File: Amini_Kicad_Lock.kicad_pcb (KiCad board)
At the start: 2 copper layers, 36 parts, among them U1 nRF5340-QKxx, X1 32MHz, X2 32.768kHz

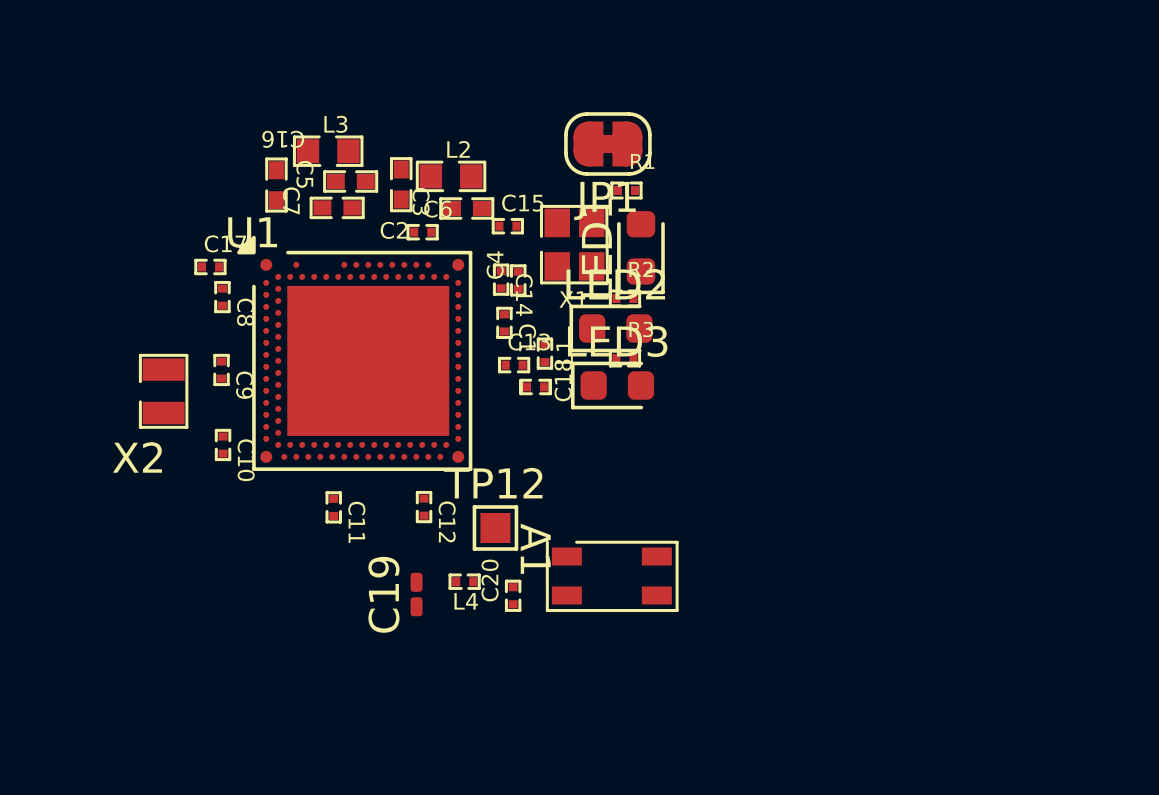
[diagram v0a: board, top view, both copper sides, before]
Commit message: 2. commit
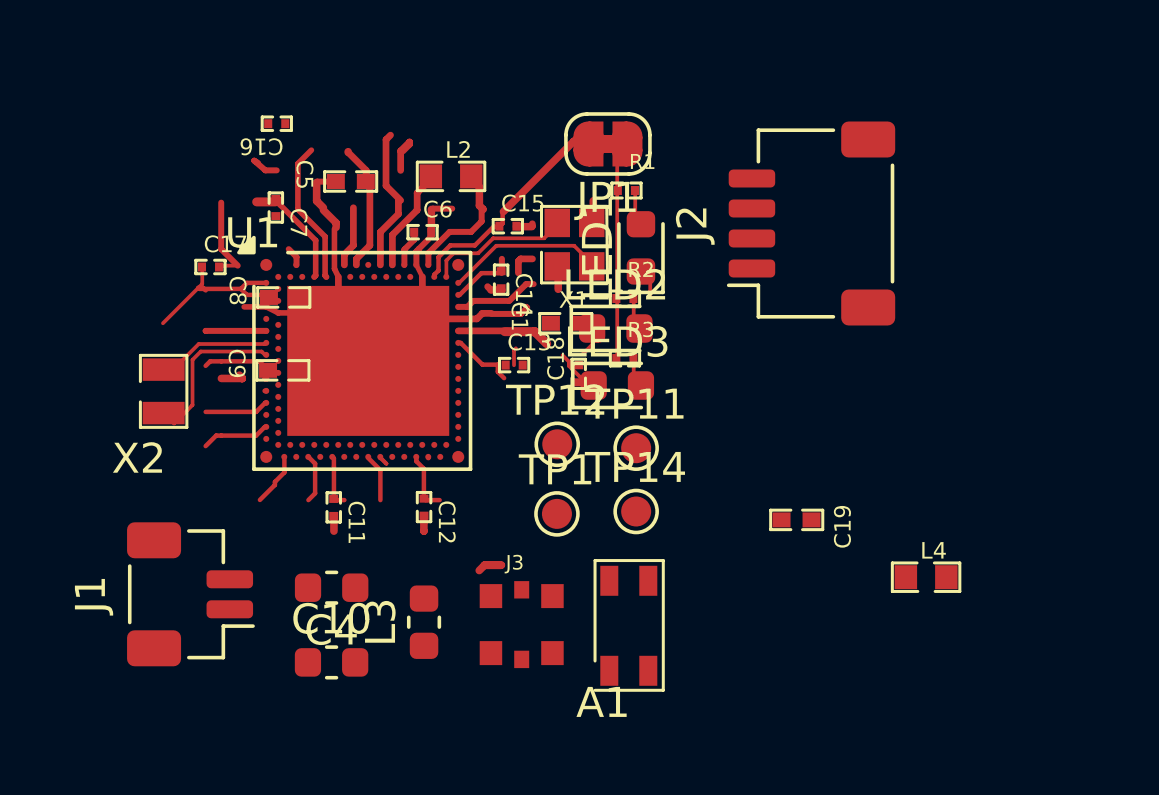
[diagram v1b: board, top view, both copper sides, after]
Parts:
- removed C2, C3: 1.0µF, Nordic_Semiconductor:CAPC1005X04L
- removed C20: 0.5pF, Nordic_Semiconductor:CAPC0603X03L_C
- removed L1: 2.2nH, Nordic_Semiconductor:INDC0603X03L_C
- added J1: Conn_01x02, Connector_JST:JST_SH_BM02B-SRSS-TB_1x02-1MP_P1.00mm_Vertical, F.Cu at (110.8, 74.4)
- added J2: Conn_01x04, Connector_JST:JST_SH_SM04B-SRSS-TB_1x04-1MP_P1.00mm_Horizontal, F.Cu at (131.5, 62.0)
- added J3: MM8130-2600RA2, MM8130-2600RA2 antenna:MURATA_MM8130-2600RA2, F.Cu at (121.9, 75.4)
- added TP1: TestPoint, TestPoint:TestPoint_Pad_D1.0mm, F.Cu at (123.0, 71.7)
- added TP11: TestPoint, TestPoint:TestPoint_Pad_D1.0mm, F.Cu at (125.7, 69.5)
- added TP14: TestPoint, TestPoint:TestPoint_Pad_D1.0mm, F.Cu at (125.7, 71.6)
- C1: value 0.7pF -> 1.0µF; footprint Nordic_Semiconductor:CAPC0603X03L_C -> Nordic_Semiconductor:CAPC1005X04L
- C10: value 100nF -> 0.7pF; footprint Nordic_Semiconductor:CAPC0603X03L_C -> Inductor_SMD:L_0603_1608Metric
- C16: value 1.0µF -> 100nF; footprint Nordic_Semiconductor:CAPC1005X04L -> Nordic_Semiconductor:CAPC0603X03L_C
- C18: value N.C. -> 100nF; footprint Nordic_Semiconductor:CAPC0603X03L_C_NC -> Nordic_Semiconductor:CAPC0603X03L_C
- C19: value N.C. -> 1.0µF; footprint Capacitor_SMD:C_0201_0603Metric_Pad0.64x0.40mm_HandSolder -> Nordic_Semiconductor:CAPC1005X04L
- C4: value 2.2nF -> N.C.; footprint Nordic_Semiconductor:CAPC0603X03L_C -> Inductor_SMD:L_0603_1608Metric
- C7: value 1.0µF -> 2.2nF; footprint Nordic_Semiconductor:CAPC1005X04L -> Nordic_Semiconductor:CAPC0603X03L_C
- C8, C9: value 100nF -> 1.0µF; footprint Nordic_Semiconductor:CAPC0603X03L_C -> Nordic_Semiconductor:CAPC1005X04L
- L3: value 10µH -> 2.2nH; footprint Nordic_Semiconductor:INDC1608X06L -> Inductor_SMD:L_0603_1608Metric
- L4: value 3.3nH -> 10µH; footprint Nordic_Semiconductor:INDC0603X03L_C -> Nordic_Semiconductor:INDC1608X06L
- TP12: footprint TestPoint:TestPoint_Pad_1.0x1.0mm -> TestPoint:TestPoint_Pad_D1.0mm
- moved L4 15.6 mm to (135.6, 74.9)
- moved L3 14.9 mm to (118.6, 75.3), turned to 90 degrees
- moved C19 14.9 mm to (133.1, 72.1)
- moved C4 11.8 mm to (115.5, 74.2), turned to 180 degrees
- moved C10 8.29 mm to (115.5, 76.7), turned to 0 degrees
- moved A1 6.24 mm to (124.6, 78.5), turned to 0 degrees
- moved TP12 3.47 mm to (123.0, 69.4)
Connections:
- C1 pad 1: GND -> VDD_nRF
- C1 pad 2: Net-(U1-ANT) -> GND
- C10 pad 1: VDD_nRF -> GND
- C10 pad 2: GND -> Net-(U1-ANT)
- C16 pad 1: GND -> VDD_nRF
- C16 pad 2: VDD_nRF -> GND
- C18 pad 1: GND -> VDD_nRF
- C18 pad 2: (no net) -> GND
- C19 pad 2: (no net) -> VDD_nRF
- C4 pad 1: Net-(U1-DECR) -> GND
- C4 pad 2: GND -> Net-(C4-Pad2)
- C5 pad 2: Net-(U1-DECD) -> Net-(U1-DECR)
- C7 pad 1: GND -> Net-(U1-DECR)
- C7 pad 2: Net-(U1-DECA) -> GND
- C8 pad 1: VDD_nRF -> GND
- C8 pad 2: GND -> Net-(U1-DECD)
- C9 pad 1: VDD_nRF -> GND
- C9 pad 2: GND -> Net-(U1-DECA)
- L3 pad 1: Net-(U1-DECD) -> Net-(U1-ANT)
- L3 pad 2: Net-(U1-DCCD) -> Net-(C4-Pad2)
- L4 pad 1: Net-(A1-Pad1) -> Net-(U1-DECD)
- L4 pad 2: (no net) -> Net-(U1-DCCD)
- TP12 pad 1: (no net) -> /SWDIO
- U1 pad AK10: (no net) -> unconnected-(U1-IO2/P0.15-PadAK10)
- U1 pad AK12: (no net) -> unconnected-(U1-SCK/P0.17-PadAK12)
- U1 pad AK14: (no net) -> unconnected-(U1-CSN/P0.18-PadAK14)
- U1 pad AK30: (no net) -> unconnected-(U1-AIN6/P0.27-PadAK30)
- U1 pad AK8: (no net) -> unconnected-(U1-IO1/P0.14-PadAK8)
- U1 pad AL27: (no net) -> unconnected-(U1-P0.24-PadAL27)
- U1 pad AL29: (no net) -> unconnected-(U1-AIN5/P0.26-PadAL29)
- U1 pad AL5: (no net) -> unconnected-(U1-IO0/P0.13-PadAL5)
- U1 pad AL9: (no net) -> unconnected-(U1-IO3/P0.16-PadAL9)
- U1 pad B22: (no net) -> unconnected-(U1-P0.31-PadB22)
- U1 pad G1: GND -> unconnected-(U1-NC-PadG1)
- U1 pad H2: GND -> unconnected-(U1-NC-PadH2)
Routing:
- net VDD_nRF: track 0.00 -> 45.9 mm
- net GND: track 0.00 -> 24.6 mm
- net Net-(JP1-A): track 0.00 -> 7.26 mm
- net Net-(U1-DECR): track 0.00 -> 7.00 mm
- net Net-(U1-DECD): track 0.00 -> 5.65 mm
- net Net-(U1-XL2/P0.01): track 0.00 -> 5.35 mm
- net /XC1: track 0.00 -> 5.35 mm
- net /XC2: track 0.00 -> 4.81 mm
- net Net-(U1-DCCD): track 0.00 -> 4.80 mm
- net Net-(U1-XL1/P0.00): track 0.00 -> 3.79 mm
- net Net-(U1-DCC): track 0.00 -> 3.41 mm
- net Net-(U1-ANT): track 0.00 -> 3.21 mm
- net Net-(U1-DECA): track 0.00 -> 2.88 mm
- net /P0.30: track 0.00 -> 1.55 mm
- net Net-(A1-Pad1): track 0.00 -> 1.46 mm
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
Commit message: 3. commit
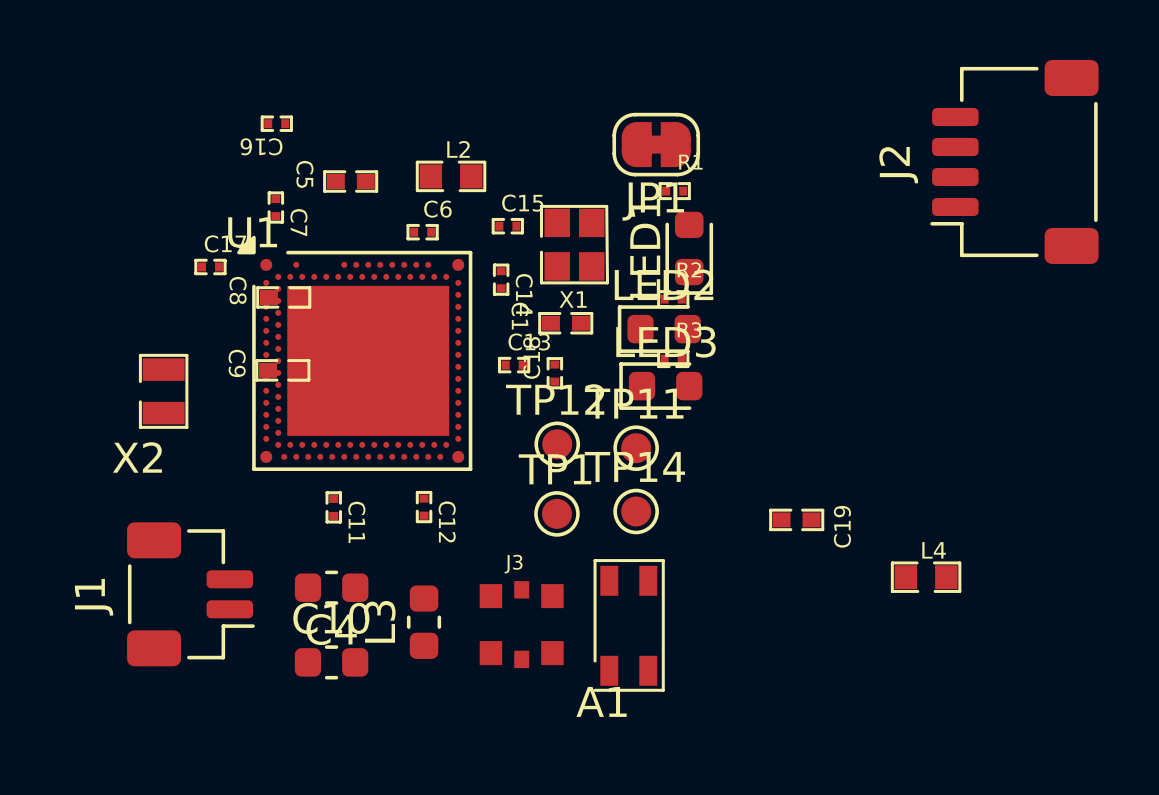
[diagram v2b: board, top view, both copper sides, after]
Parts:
- moved J2 7.08 mm to (138.3, 60.0)
- moved JP1 1.61 mm to (126.3, 59.4)
- moved LED1 1.61 mm to (127.5, 62.9)
- moved LED2 1.61 mm to (126.6, 65.5)
- moved LED3 1.61 mm to (126.7, 67.4)
- moved R1 1.61 mm to (126.9, 61.1)
- moved R2 1.61 mm to (126.9, 64.7)
- moved R3 1.61 mm to (126.9, 66.7)
- moved C18 0.80 mm to (123.0, 67.2)
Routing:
- net VDD_nRF: track 45.9 -> 0.00 mm
- net GND: track 24.6 -> 0.00 mm
- net Net-(JP1-A): track 7.26 -> 0.00 mm
- net Net-(U1-DECR): track 7.00 -> 0.00 mm
- net Net-(U1-DECD): track 5.65 -> 0.00 mm
- net Net-(U1-XL2/P0.01): track 5.35 -> 0.00 mm
- net /XC1: track 5.35 -> 0.00 mm
- net /XC2: track 4.81 -> 0.00 mm
- net Net-(U1-DCCD): track 4.80 -> 0.00 mm
- net Net-(U1-XL1/P0.00): track 3.79 -> 0.00 mm
- net Net-(U1-DCC): track 3.41 -> 0.00 mm
- net Net-(U1-ANT): track 3.21 -> 0.00 mm
- net Net-(U1-DECA): track 2.88 -> 0.00 mm
- net /P0.30: track 1.55 -> 0.00 mm
- net Net-(A1-Pad1): track 1.46 -> 0.00 mm
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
